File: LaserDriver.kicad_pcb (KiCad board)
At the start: 2 copper layers, 40 x 40 mm, 31 parts, among them J100 Screw_Terminal_01x04, J101 Screw_Terminal_01x02, J102 nano_left, J103 nano_right, U100 TPS92513DGQR

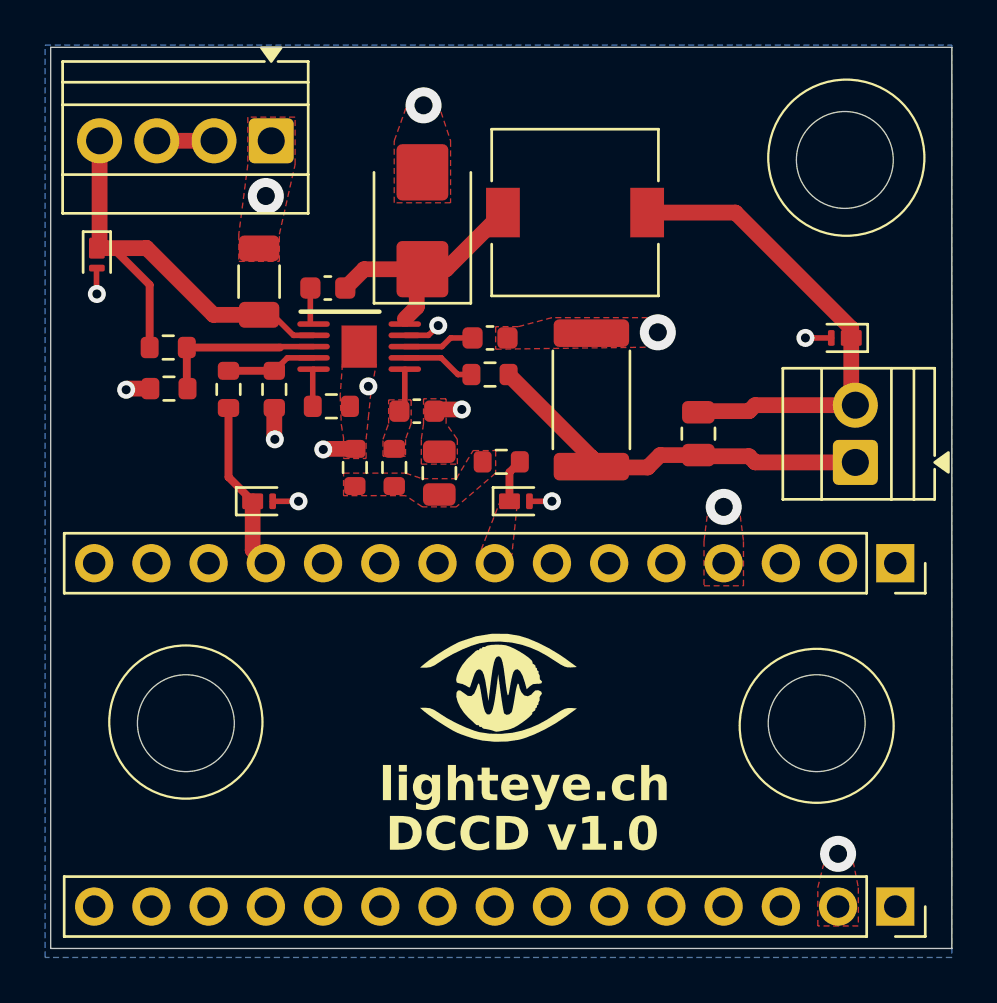
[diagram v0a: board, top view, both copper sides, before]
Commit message: fine changes
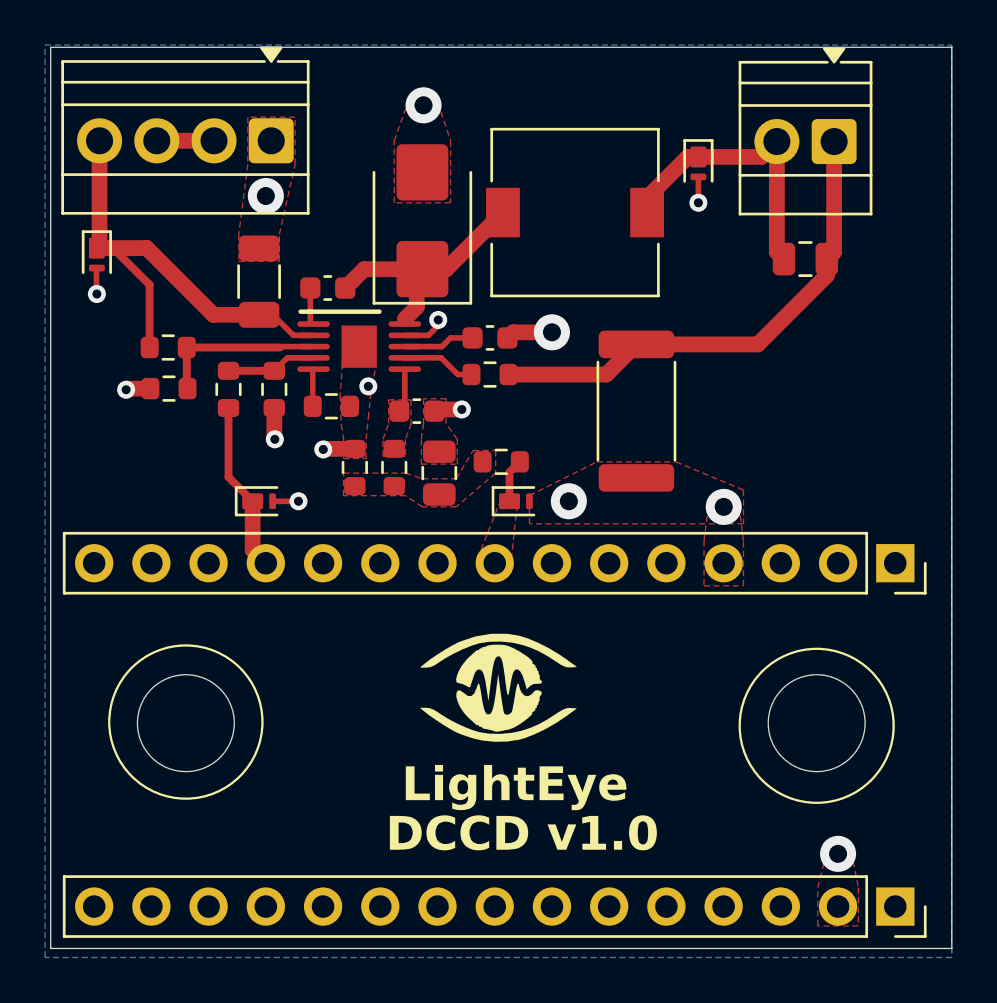
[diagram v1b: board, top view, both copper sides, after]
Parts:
- removed H2: MountingHole, MountingHole:MountingHole_4.3mm_M4
- moved J101 14.3 mm to (64.5, 101.3), turned to 180 degrees
- moved D102 10.1 mm to (58.5, 102.2), turned to -90 degrees
- moved C104 9.09 mm to (63.2, 106.5), turned to 0 degrees
- moved R105 2.06 mm to (55.8, 113.2), turned to -90 degrees
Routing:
- net Net-(D102-K): track 21.8 -> 12.8 mm
- net Net-(J101-Pin_1): track 18.1 -> 22.0 mm
- net GND: track 12.8 -> 13.9 mm
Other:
- board text added: "LightEye"
- board text removed: "lighteye.ch"
